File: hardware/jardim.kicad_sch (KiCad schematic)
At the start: 91 parts, among them J1 DC_INPUT, J10 DHT22_AMB, J11 LIGHT_SENSOR_1, J12 LIGHT_SENSOR_2, J13 LEVEL_SENSOR_1, J14 LEVEL_SENSOR_2, J15 SOIL_HUMIDITY_SENSOR_1, J16 SOIL_HUMIDITY_SENSOR_2, J18 USB_C_Receptacle_PowerOnly_6P, J2 PUMP_1, J3 PUMP_2, J4 LIGHT_1, J5 LIGHG_2, J6 HEAT_1, J7 HEAT_2, J8 DS12B20_2, J9 DS18B20_1, Q1 FQP30N06L, Q2 FQP30N06L, Q3 FQP30N06L, Q4 FQP30N06L, Q5 FQP30N06L, Q6 FQP30N06L, Q7 BC337, SW1 SW_Push, SW2 SW_Push, SW3 SW_Push, SW4 SW_SPST, U1 AM2302, U2 DM-OLED096-636

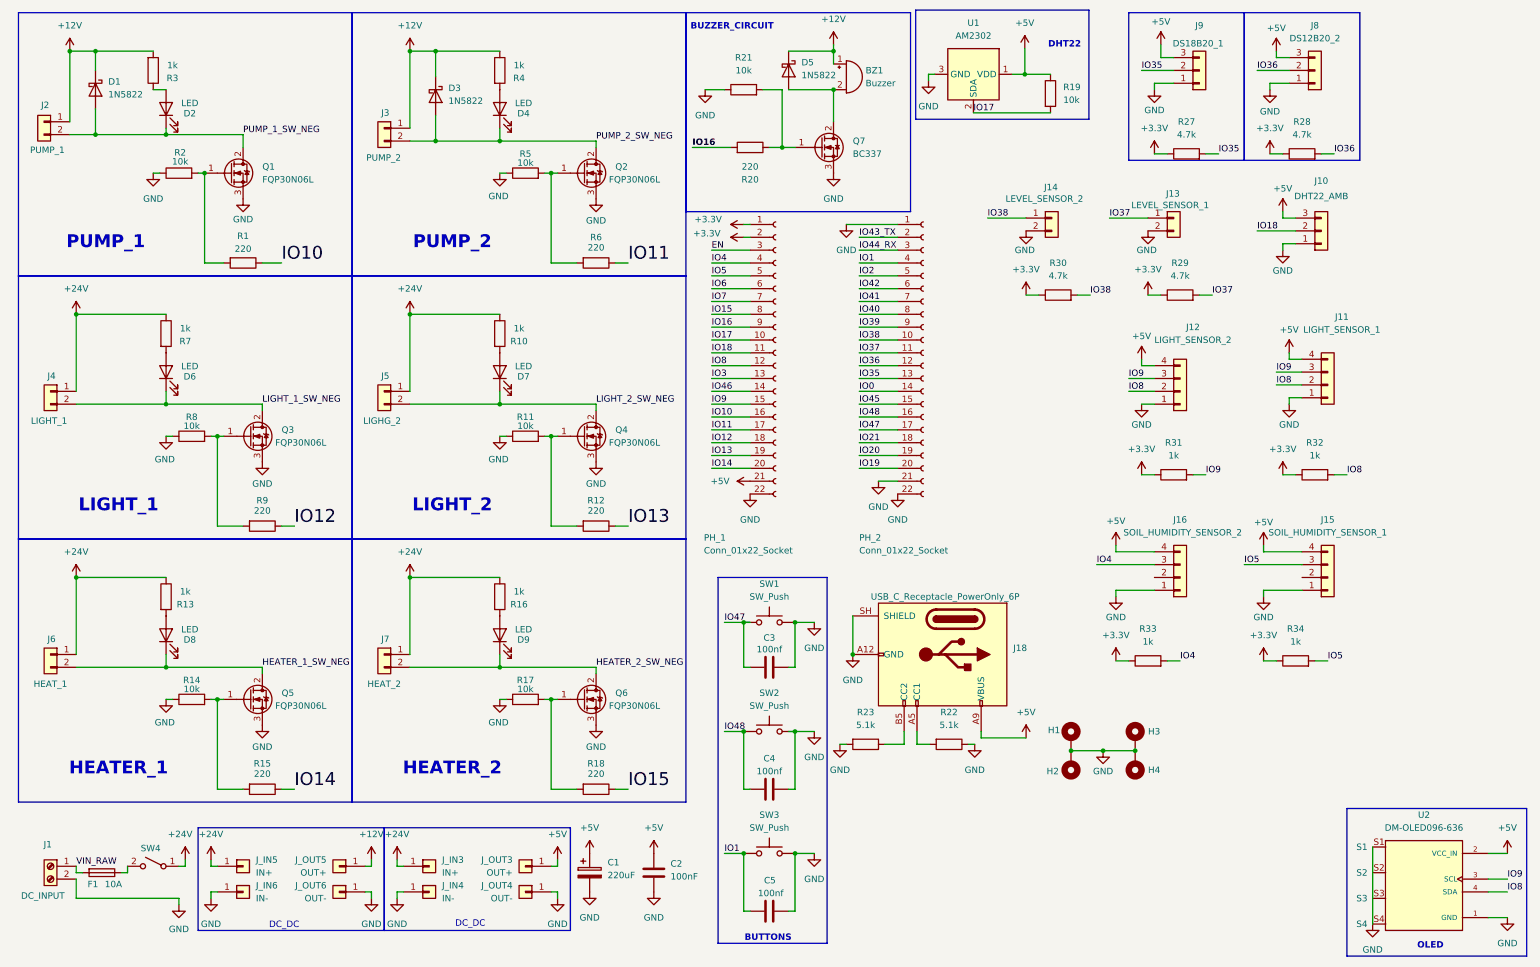
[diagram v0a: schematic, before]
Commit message: ajustes
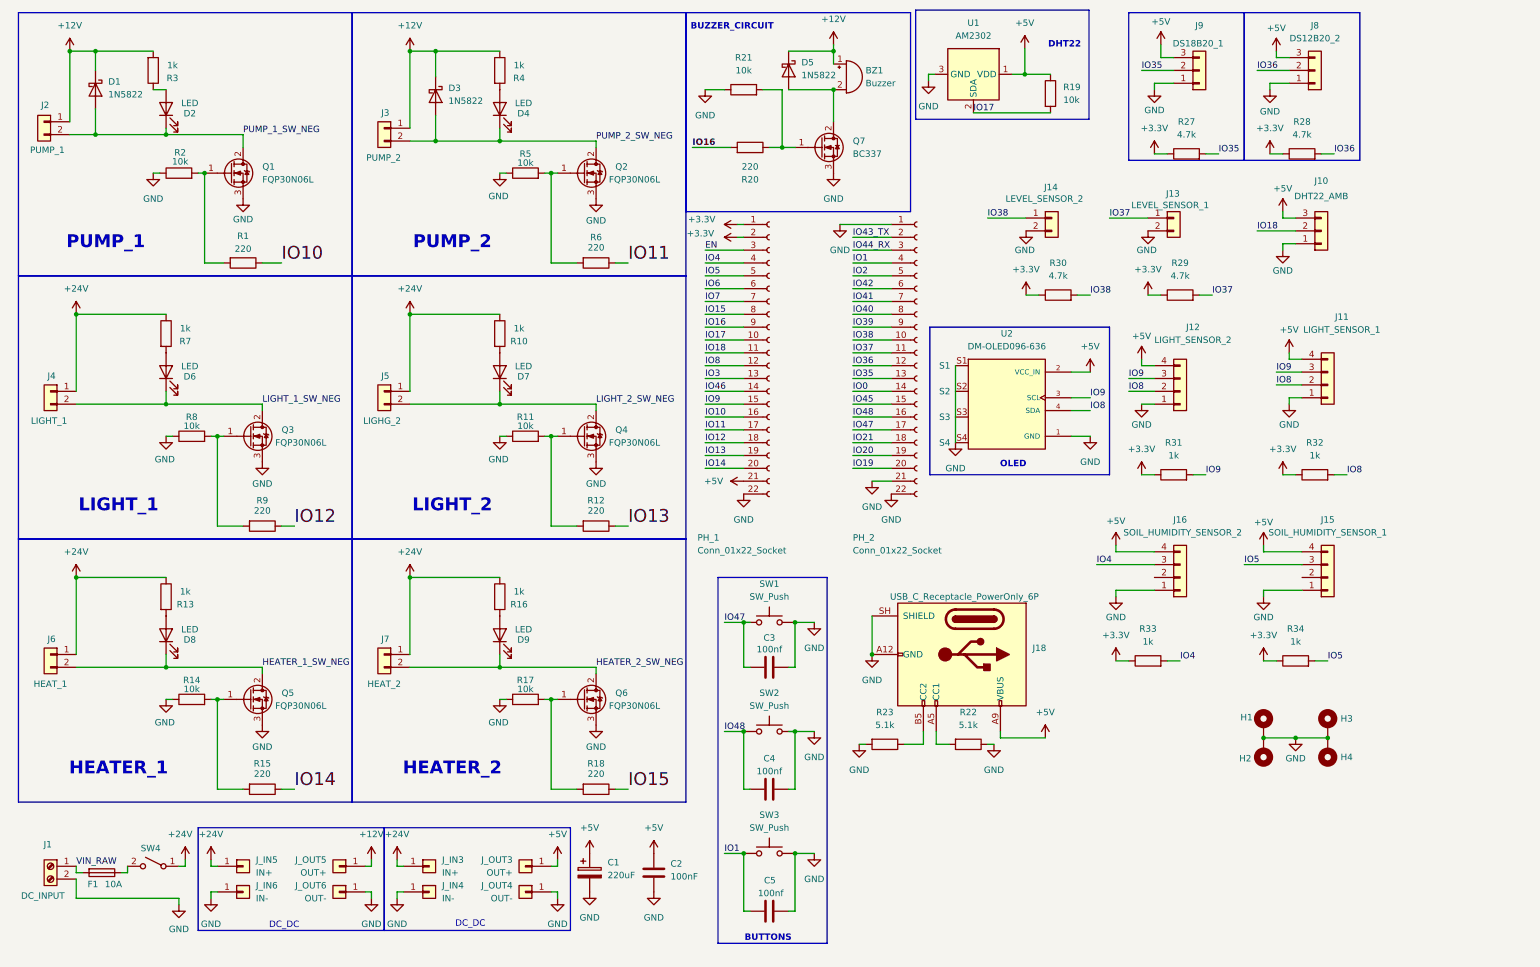
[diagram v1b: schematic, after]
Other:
- moved on the sheet: H1, H2, H3, H4, J18, PH_1, PH_2, R22, R23, U2

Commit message: sem avisos, pronto para rotear
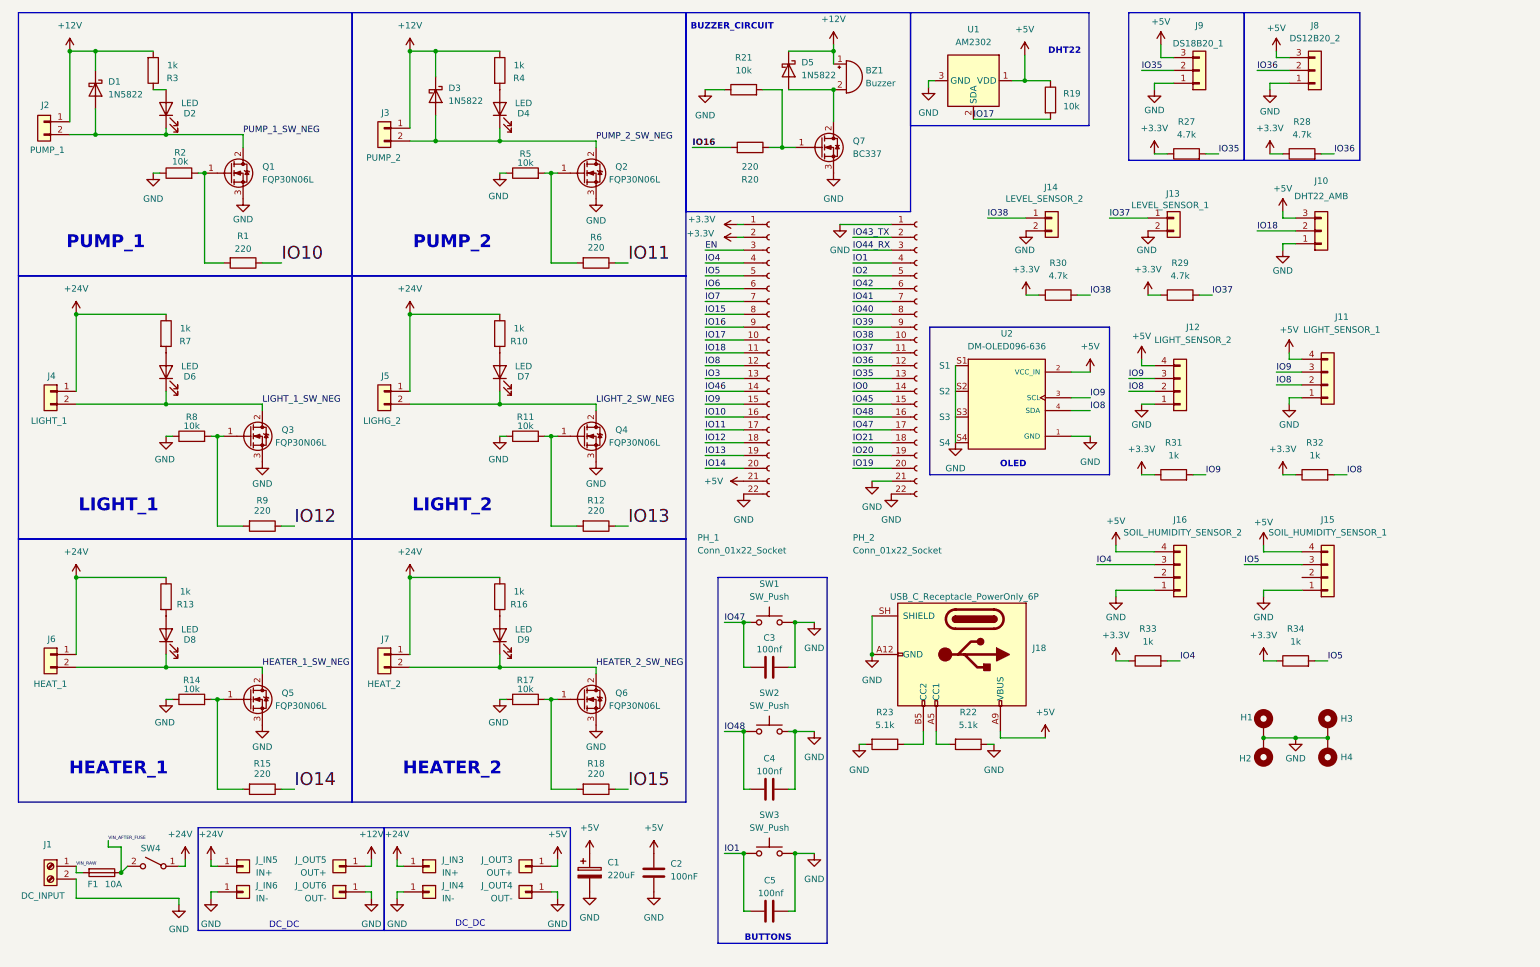
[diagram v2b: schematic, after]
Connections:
- net VIN_AFTER_FUSE: now reaches F1.1, SW4.2 (B)
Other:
- moved on the sheet: R19, U1
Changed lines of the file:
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@@
 	)
 	(rectangle
-		(start 190.246 12.192)
-		(end 224.536 33.782)
+		(start 189.23 12.7)
+		(end 224.536 35.052)
 		(stroke
 			(width 0)
@@
 	(text "DHT22"
 		(exclude_from_sim no)
-		(at 219.71 19.05 0)
+		(at 219.71 20.32 0)
 		(effects
 			(font
@@
 	)
 	(junction
+		(at 33.02 182.88)
+		(diameter 0)
+		(color 0 0 0 0)
+	)
+	(junction
 		(at 173.99 20.32)
 		(diameter 0)
@@
 	)
 	(junction
-		(at 211.836 24.892)
+		(at 211.836 26.162)
 		(diameter 0)
 		(color 0 0 0 0)
@@
 	(wire
 		(pts
-			(xy 34.29 182.88) (xy 33.02 182.88)
-		)
-		(stroke
-			(width 0)
-			(type default)
-		)
-	)
-	(wire
-		(pts
 			(xy 27.94 20.32) (xy 27.94 24.13)
 		)
@@
 	(wire
 		(pts
-			(xy 194.056 24.892) (xy 192.786 24.892)
+			(xy 194.056 26.162) (xy 192.786 26.162)
 		)
 		(stroke
@@
 	(wire
 		(pts
+			(xy 33.02 182.88) (xy 34.29 181.61)
+		)
+		(stroke
+			(width 0)
+			(type default)
+		)
+	)
+	(wire
+		(pts
 			(xy 264.16 81.28) (xy 266.7 81.28)
 		)
@@
 	(wire
 		(pts
-			(xy 192.786 24.892) (xy 192.786 26.162)
+			(xy 192.786 26.162) (xy 192.786 27.432)
 		)
 		(stroke
@@
 	(wire
 		(pts
-			(xy 211.836 19.812) (xy 211.836 24.892)
+			(xy 211.836 21.082) (xy 211.836 26.162)
 		)
 		(stroke
@@
 	(wire
 		(pts
-			(xy 201.676 32.512) (xy 216.916 32.512)
+			(xy 201.676 33.782) (xy 216.916 33.782)
 		)
 		(stroke
@@
 	(wire
 		(pts
+			(xy 30.48 177.8) (xy 33.02 177.8)
+		)
+		(stroke
+			(width 0)
+			(type default)
+		)
+	)
+	(wire
+		(pts
 			(xy 45.72 180.34) (xy 45.72 181.61)
 		)
@@
 	(wire
 		(pts
+			(xy 30.48 176.53) (xy 30.48 177.8)
+		)
+		(stroke
+			(width 0)
+			(type default)
+		)
+	)
+	(wire
+		(pts
 			(xy 90.17 20.32) (xy 90.17 35.56)
 		)
@@
 	(wire
 		(pts
-			(xy 34.29 182.88) (xy 34.29 181.61)
-		)
-		(stroke
-			(width 0)
-			(type default)
-		)
-	)
-	(wire
-		(pts
 			(xy 148.59 87.63) (xy 156.21 87.63)
 		)
@@
 	(wire
 		(pts
+			(xy 33.02 177.8) (xy 33.02 182.88)
+		)
+		(stroke
+			(width 0)
+			(type default)
+		)
+	)
+	(wire
+		(pts
 			(xy 257.81 24.13) (xy 264.16 24.13)
 		)
@@
 	(wire
 		(pts
-			(xy 209.296 24.892) (xy 211.836 24.892)
+			(xy 209.296 26.162) (xy 211.836 26.162)
 		)
 		(stroke
@@
 	(wire
 		(pts
-			(xy 211.836 24.892) (xy 216.916 24.892)
+			(xy 211.836 26.162) (xy 216.916 26.162)
 		)
 		(stroke
@@
 	)
 	(label "IO17"
-		(at 201.676 32.512 0)
+		(at 201.676 33.782 0)
 		(effects
 			(font
@@
 		(effects
 			(font
-				(size 1.27 1.27)
+				(size 0.635 0.635)
 			)
 			(justify left bottom)
@@
 		)
 	)
+	(label "VIN_AFTER_FUSE"
+		(at 30.48 176.53 0)
+		(effects
+			(font
+				(size 0.635 0.635)
+			)
+			(justify left bottom)
+		)
+	)
 	(label "IO35"
 		(at 250.19 40.64 0)
@@
 	(symbol
 		(lib_id "Sensor:AM2302")
-		(at 201.676 24.892 270)
+		(at 201.676 26.162 270)
 		(unit 1)
 		(body_style 1)
@@
 		(fields_autoplaced yes)
 		(property "Reference" "U1"
-			(at 201.676 14.732 90)
+			(at 201.676 16.002 90)
 			(show_name no)
 			(do_not_autoplace no)
@@
 		)
 		(property "Value" "AM2302"
-			(at 201.676 17.272 90)
+			(at 201.676 18.542 90)
 			(show_name no)
 			(do_not_autoplace no)
@@
 		)
 		(property "Footprint" "Sensor:ASAIR_AM2302_P2.54mm_Vertical"
-			(at 191.516 24.892 0)
+			(at 191.516 26.162 0)
 			(hide yes)
 			(show_name no)
@@
 		)
 		(property "Datasheet" "http://akizukidenshi.com/download/ds/aosong/AM2302.pdf"
-			(at 208.026 28.702 0)
+			(at 208.026 29.972 0)
 			(hide yes)
 			(show_name no)
@@
 		)
 		(property "Description" "3.3 to 5.0V, Temperature and humidity module,  DHT22, AM2302"
-			(at 201.676 24.892 0)
+			(at 201.676 26.162 0)
 			(hide yes)
 			(show_name no)
@@
 	(symbol
 		(lib_id "power:+5V")
-		(at 211.836 19.812 0)
+		(at 211.836 21.082 0)
 		(unit 1)
 		(body_style 1)
@@
 		(fields_autoplaced yes)
 		(property "Reference" "#PWR039"
-			(at 211.836 23.622 0)
+			(at 211.836 24.892 0)
 			(hide yes)
 			(show_name no)
@@
 		)
 		(property "Value" "+5V"
-			(at 211.836 14.732 0)
+			(at 211.836 16.002 0)
 			(show_name no)
 			(do_not_autoplace no)
@@
 		)
 		(property "Footprint" ""
-			(at 211.836 19.812 0)
+			(at 211.836 21.082 0)
 			(hide yes)
 			(show_name no)
@@
 		)
 		(property "Datasheet" ""
-			(at 211.836 19.812 0)
+			(at 211.836 21.082 0)
 			(hide yes)
 			(show_name no)
@@
 		)
 		(property "Description" "Power symbol creates a global label with name \"+5V\""
-			(at 211.836 19.812 0)
+			(at 211.836 21.082 0)
 			(hide yes)
 			(show_name no)
@@
 	(symbol
 		(lib_id "Device:R")
-		(at 216.916 28.702 0)
+		(at 216.916 29.972 0)
 		(unit 1)
 		(body_style 1)
@@
 		(fields_autoplaced yes)
 		(property "Reference" "R19"
-			(at 219.456 27.4319 0)
+			(at 219.456 28.7019 0)
 			(show_name no)
 			(do_not_autoplace no)
@@
 		)
 		(property "Value" "10k"
-			(at 219.456 29.9719 0)
+			(at 219.456 31.2419 0)
 			(show_name no)
 			(do_not_autoplace no)
@@
 		)
 		(property "Footprint" "Resistor_THT:R_Axial_DIN0207_L6.3mm_D2.5mm_P7.62mm_Horizontal"
-			(at 215.138 28.702 90)
+			(at 215.138 29.972 90)
 			(hide yes)
 			(show_name no)
@@
 		)
 		(property "Datasheet" ""
-			(at 216.916 28.702 0)
+			(at 216.916 29.972 0)
 			(hide yes)
 			(show_name no)
@@
 		)
 		(property "Description" "Resistor"
-			(at 216.916 28.702 0)
+			(at 216.916 29.972 0)
 			(hide yes)
 			(show_name no)
@@
 	(symbol
 		(lib_id "power:GND")
-		(at 192.786 26.162 0)
+		(at 192.786 27.432 0)
 		(unit 1)
 		(body_style 1)
@@
 		(fields_autoplaced yes)
 		(property "Reference" "#PWR038"
-			(at 192.786 32.512 0)
+			(at 192.786 33.782 0)
 			(hide yes)
 			(show_name no)
@@
 		)
 		(property "Value" "GND"
-			(at 192.786 31.242 0)
+			(at 192.786 32.512 0)
 			(show_name no)
 			(do_not_autoplace no)
@@
 		)
 		(property "Footprint" ""
-			(at 192.786 26.162 0)
+			(at 192.786 27.432 0)
 			(hide yes)
 			(show_name no)
@@
 		)
 		(property "Datasheet" ""
-			(at 192.786 26.162 0)
+			(at 192.786 27.432 0)
 			(hide yes)
 			(show_name no)
@@
 		)
 		(property "Description" "Power symbol creates a global label with name \"GND\" , ground"
-			(at 192.786 26.162 0)
+			(at 192.786 27.432 0)
 			(hide yes)
 			(show_name no)
@@
 	)
 	(group ""
+		(members "36834f7f-8285-48e7-a18e-6709d078e4f1" "43618f34-a686-4c66-a7ac-3ed4bba3929d"
+			"9b582545-4161-429e-9acc-5a08f32a2e5a"
+		)
+	)
+	(group ""
 		(members "20d06328-826c-48b3-8cdf-d8901b22d23b" "24e0ce1e-2f5c-4474-b50c-ba1d36bf0a1a"
 			"251f320c-7bdf-486d-b8a6-300ae3def773" "702d38d7-4511-4241-94b6-c4c3d68f2b39"
@@
 		)
 	)
-	(group ""
-		(members "36834f7f-8285-48e7-a18e-6709d078e4f1" "43618f34-a686-4c66-a7ac-3ed4bba3929d"
-			"9b582545-4161-429e-9acc-5a08f32a2e5a"
-		)
-	)
